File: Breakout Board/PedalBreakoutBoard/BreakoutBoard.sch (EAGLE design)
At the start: 45 parts, among them U1 ES_DAISY_SEED_REV4

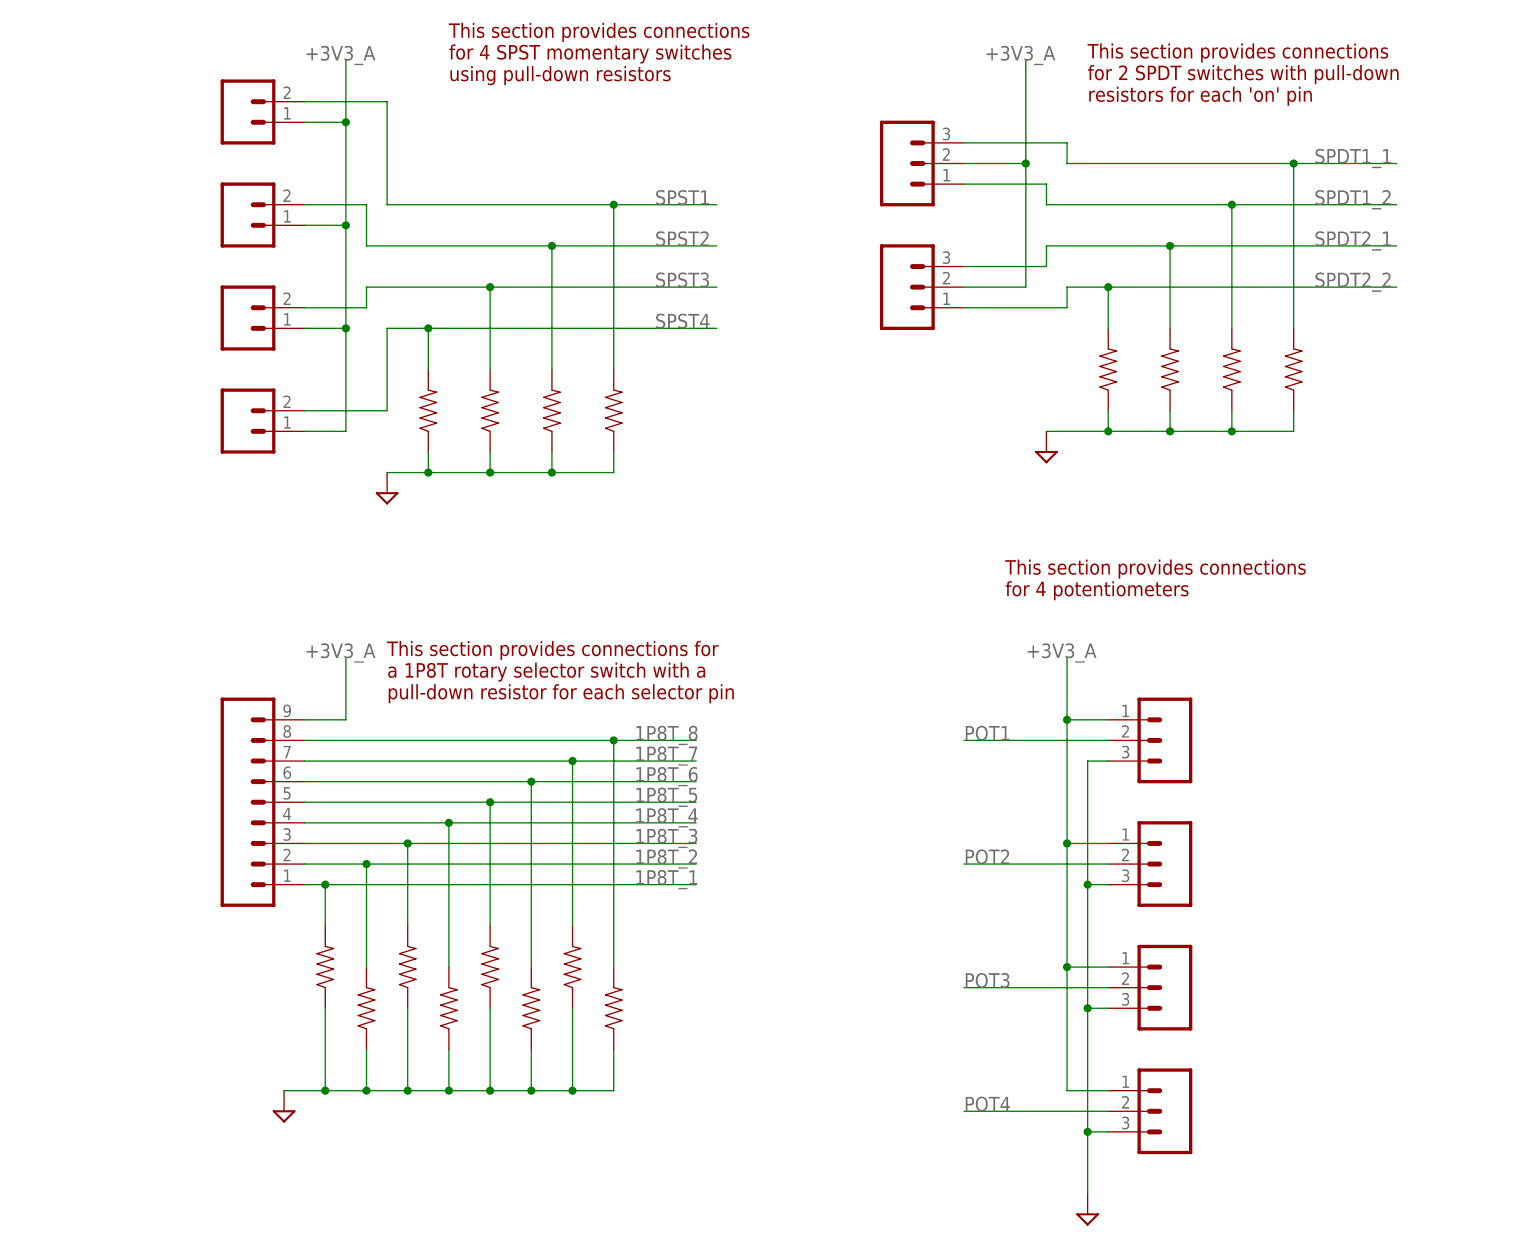
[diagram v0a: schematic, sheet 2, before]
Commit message: DP-16 - Board layout REV-A
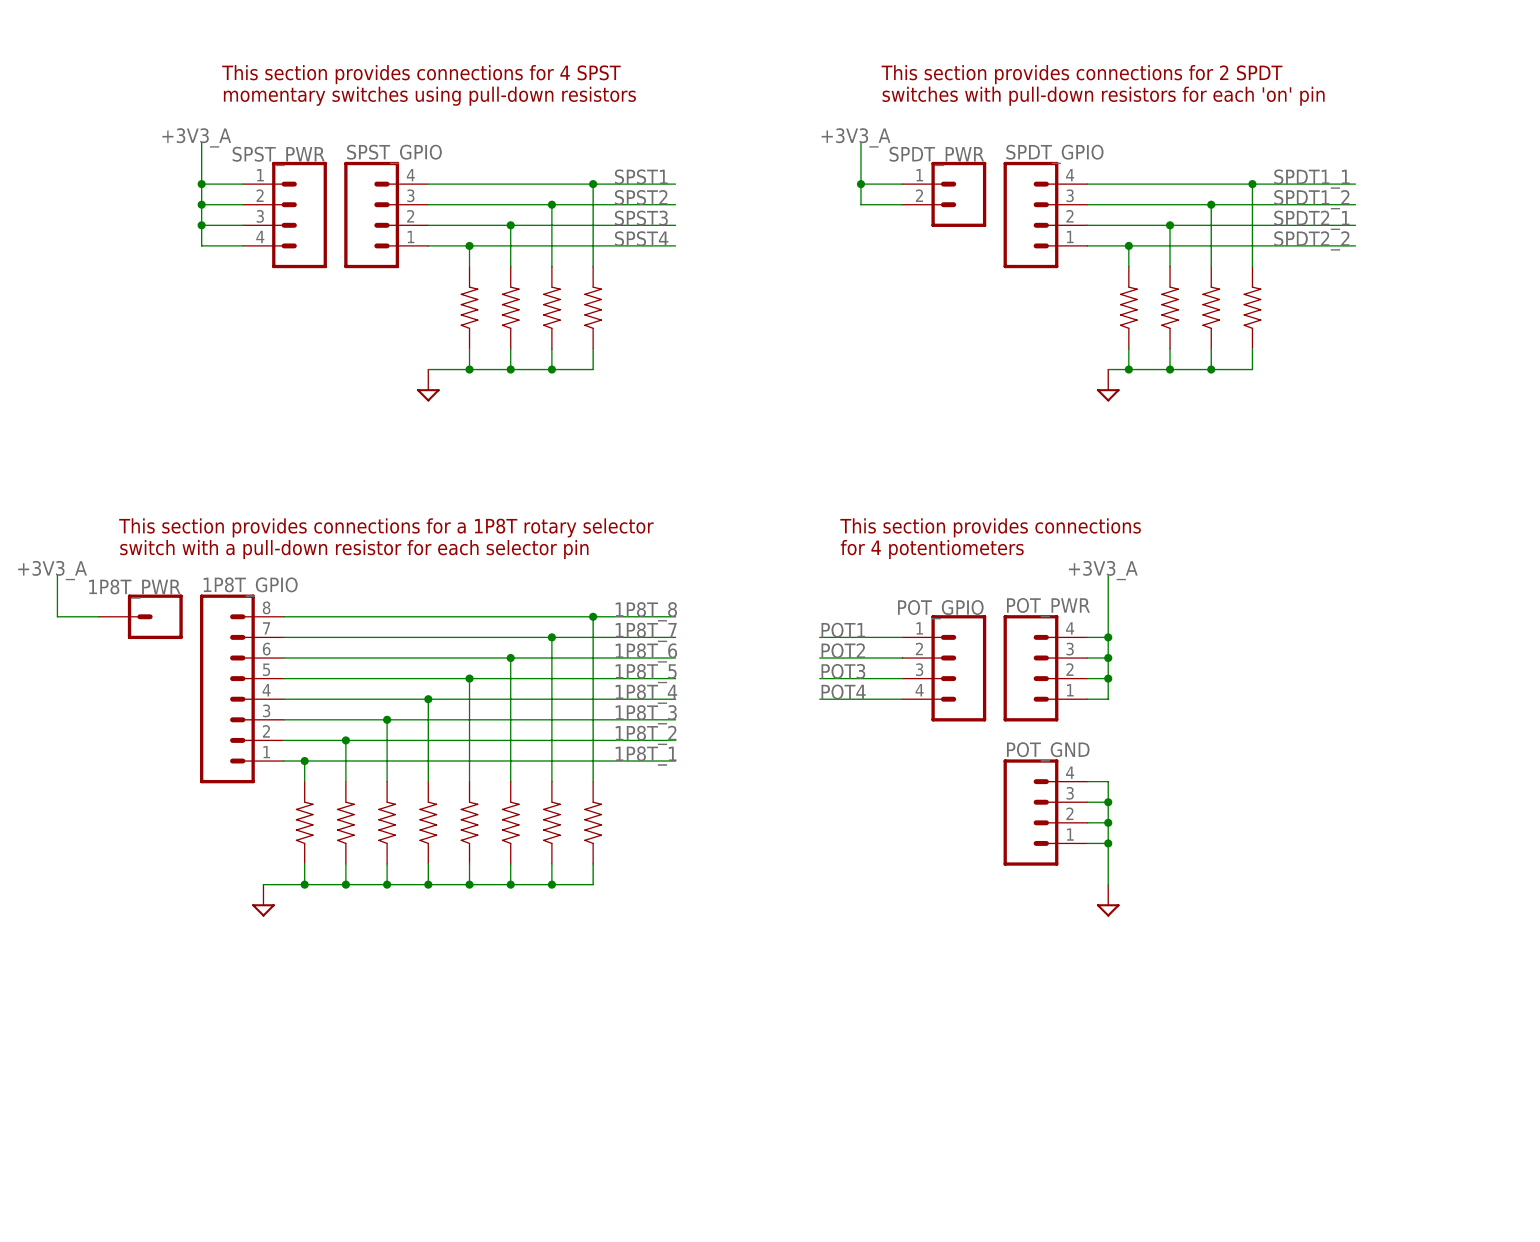
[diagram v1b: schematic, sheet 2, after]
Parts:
- removed 1P8T: (no value), SparkFun-Connectors:CONN_09
- removed GPIOS: (no value), SparkFun-Connectors:CONN_07
- removed IN_L, IN_R, LED1, LED2, LED3, LED4, OUT_L, OUT_R, SPST1, SPST2, SPST3, SPST4: (no value), SparkFun-Connectors:CONN_02
- removed POT1, POT2, POT3, POT4, SPDT1, SPDT2: (no value), SparkFun-Connectors:CONN_03
- added 1P8T_GPIO: (no value), SparkFun-Connectors:CONN_08"
- added 1P8T_PWR: (no value), SparkFun-Connectors:CONN_01
- added AUDIO, EX_GND, EX_PWR: (no value), SparkFun-Connectors:CONN_04X2
- added EX_GPIOS: (no value), SparkFun-Connectors:CONN_07
- added LED_GND, LED_GPIO, POT_GND, POT_GPIO, POT_PWR, SPDT_GPIO, SPST_GPIO, SPST_PWR: (no value), SparkFun-Connectors:CONN_04
- added SPDT_PWR: (no value), SparkFun-Connectors:CONN_02
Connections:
- removed net GPIO10: GPIOS.6, U1.GPIO10(SPI1_MISO)
- removed net GPIO11: GPIOS.5, U1.GPIO11(SPI1_MOSI)
- removed net GPIO12: GPIOS.4, U1.GPIO12(I2C1_SCL)
- removed net GPIO13: GPIOS.3, U1.GPIO13(I2C1_SDA)
- removed net GPIO14: GPIOS.2, U1.GPIO14(USART1_TX)
- removed net GPIO15: GPIOS.1, U1.GPIO15(USART1_RX)
- removed net GPIO9: GPIOS.7, U1.GPIO9(SPI1_SCK)
- removed net N$6: L2.2, LED2.1
- removed net N$7: L3.2, LED3.1
- removed net N$8: L4.2, LED4.1
- new net GPIO1: EX_GPIOS.7, U1.GPIO1(USB_HS_ID)
- new net GPIO2: EX_GPIOS.6, U1.GPIO2(SDMMC1_D3)
- new net GPIO3: EX_GPIOS.5, U1.GPIO3(SDMMC1_D2)
- new net GPIO4: EX_GPIOS.4, U1.GPIO4(SDMMC1_D1)
- new net GPIO5: EX_GPIOS.3, U1.GPIO5(SDMMC1_D0)
- new net GPIO6: EX_GPIOS.2, U1.GPIO6(SDMMC1_CMD)
- new net GPIO7: EX_GPIOS.1, U1.GPIO7(SDMMC1_CK)
- new net N$1: L1.2, LED_GPIO.1
- new net N$3: L2.2, LED_GPIO.2
- new net N$4: L3.2, LED_GPIO.3
- net +3V3_A: now also 1P8T_PWR.1, EX_PWR.1, EX_PWR.2, EX_PWR.3, EX_PWR.4, EX_PWR.5, EX_PWR.6, EX_PWR.7, EX_PWR.8, POT_PWR.1, POT_PWR.2, POT_PWR.3, POT_PWR.4, SPDT_PWR.1, SPDT_PWR.2, SPST_PWR.1, SPST_PWR.2, SPST_PWR.3, SPST_PWR.4; no longer 1P8T.9, POT1.1, POT2.1, POT3.1, POT4.1, SPDT1.2, SPDT2.2, SPST1.1, SPST2.1, SPST3.1, SPST4.1
- net 1P8T_1: now also 1P8T_GPIO.1; no longer 1P8T.1
- net 1P8T_2: now also 1P8T_GPIO.2; no longer 1P8T.2
- net 1P8T_3: now also 1P8T_GPIO.3; no longer 1P8T.3
- net 1P8T_4: now also 1P8T_GPIO.4; no longer 1P8T.4
- net 1P8T_5: now also 1P8T_GPIO.5; no longer 1P8T.5
- net 1P8T_6: now also 1P8T_GPIO.6; no longer 1P8T.6
- net 1P8T_7: now also 1P8T_GPIO.7; no longer 1P8T.7
- net 1P8T_8: now also 1P8T_GPIO.8; no longer 1P8T.8
- net GND: now also AUDIO.1, AUDIO.3, AUDIO.5, AUDIO.7, EX_GND.1, EX_GND.2, EX_GND.3, EX_GND.4, EX_GND.5, EX_GND.6, EX_GND.7, EX_GND.8, LED_GND.1, LED_GND.2, LED_GND.3, LED_GND.4, POT_GND.1, POT_GND.2, POT_GND.3, POT_GND.4; no longer IN_L.1, IN_R.1, LED1.2, LED2.2, LED3.2, LED4.2, OUT_L.1, OUT_R.1, POT1.3, POT2.3, POT3.3, POT4.3
- net IN_L: now also AUDIO.2; no longer IN_L.2
- net IN_R: now also AUDIO.4; no longer IN_R.2
- net N$5: now also L4.2, LED_GPIO.4; no longer L1.2, LED1.1
- net OUT_L: now also AUDIO.6; no longer OUT_L.2
- net OUT_R: now also AUDIO.8; no longer OUT_R.2
- net POT1: now also POT_GPIO.1; no longer POT1.2
- net POT2: now also POT_GPIO.2; no longer POT2.2
- net POT3: now also POT_GPIO.3; no longer POT3.2
- net POT4: now also POT_GPIO.4; no longer POT4.2
- net SPDT1_1: now also SPDT_GPIO.4, U1.GPIO12(I2C1_SCL); no longer SPDT1.3, U1.GPIO5(SDMMC1_D0)
- net SPDT1_2: now also SPDT_GPIO.3, U1.GPIO13(I2C1_SDA); no longer SPDT1.1, U1.GPIO6(SDMMC1_CMD)
- net SPDT2_1: now also SPDT_GPIO.2, U1.GPIO14(USART1_TX); no longer SPDT2.3, U1.GPIO7(SDMMC1_CK)
- net SPDT2_2: now also SPDT_GPIO.1, U1.GPIO15(USART1_RX); no longer SPDT2.1, U1.GPIO8(SPI1_NSS)
- net SPST1: now also SPST_GPIO.4, U1.GPIO8(SPI1_NSS); no longer SPST1.2, U1.GPIO1(USB_HS_ID)
- net SPST2: now also SPST_GPIO.3, U1.GPIO9(SPI1_SCK); no longer SPST2.2, U1.GPIO2(SDMMC1_D3)
- net SPST3: now also SPST_GPIO.2, U1.GPIO10(SPI1_MISO); no longer SPST3.2, U1.GPIO3(SDMMC1_D2)
- net SPST4: now also SPST_GPIO.1, U1.GPIO11(SPI1_MOSI); no longer SPST4.2, U1.GPIO4(SDMMC1_D1)
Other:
- moved on the sheet: L1, L2, L3, L4
